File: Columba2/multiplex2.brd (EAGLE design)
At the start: 37.7 x 35.1 mm, 19 parts, among them U1 MAX4617CUE+T

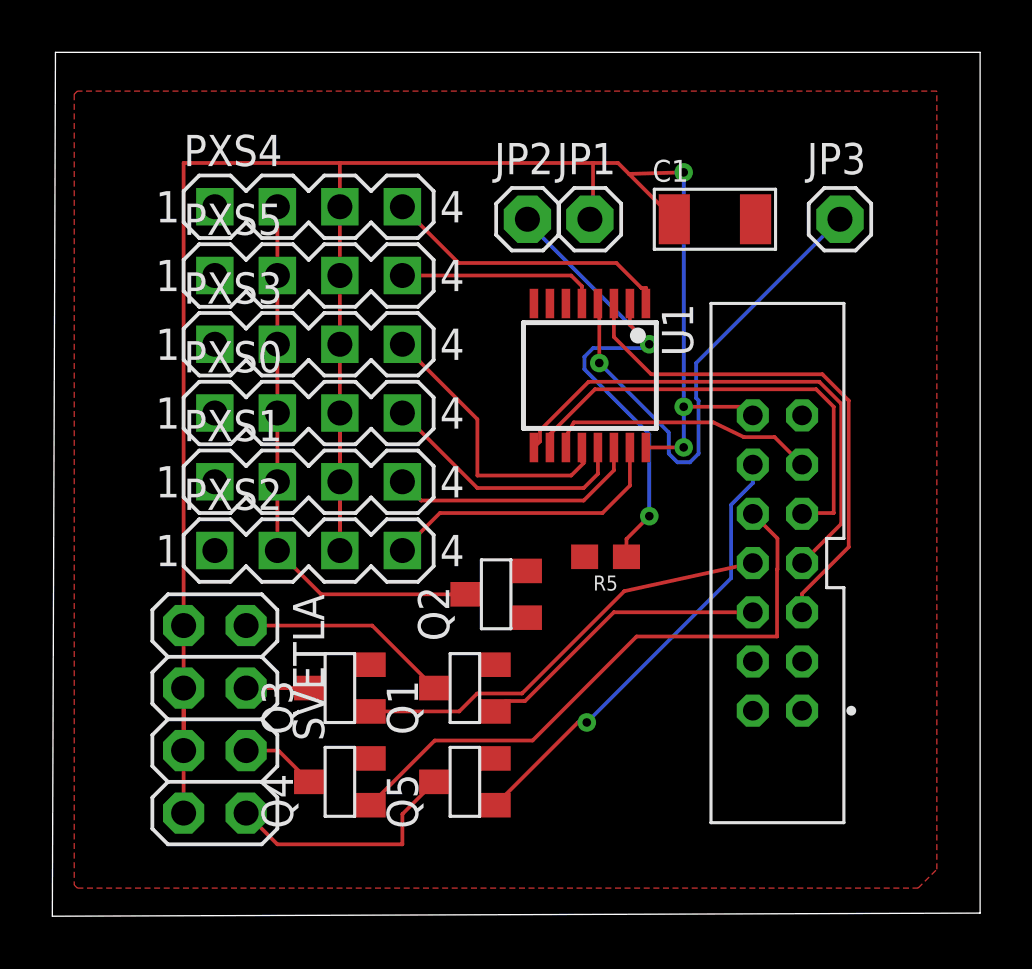
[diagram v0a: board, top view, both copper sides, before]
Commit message: Add files via upload
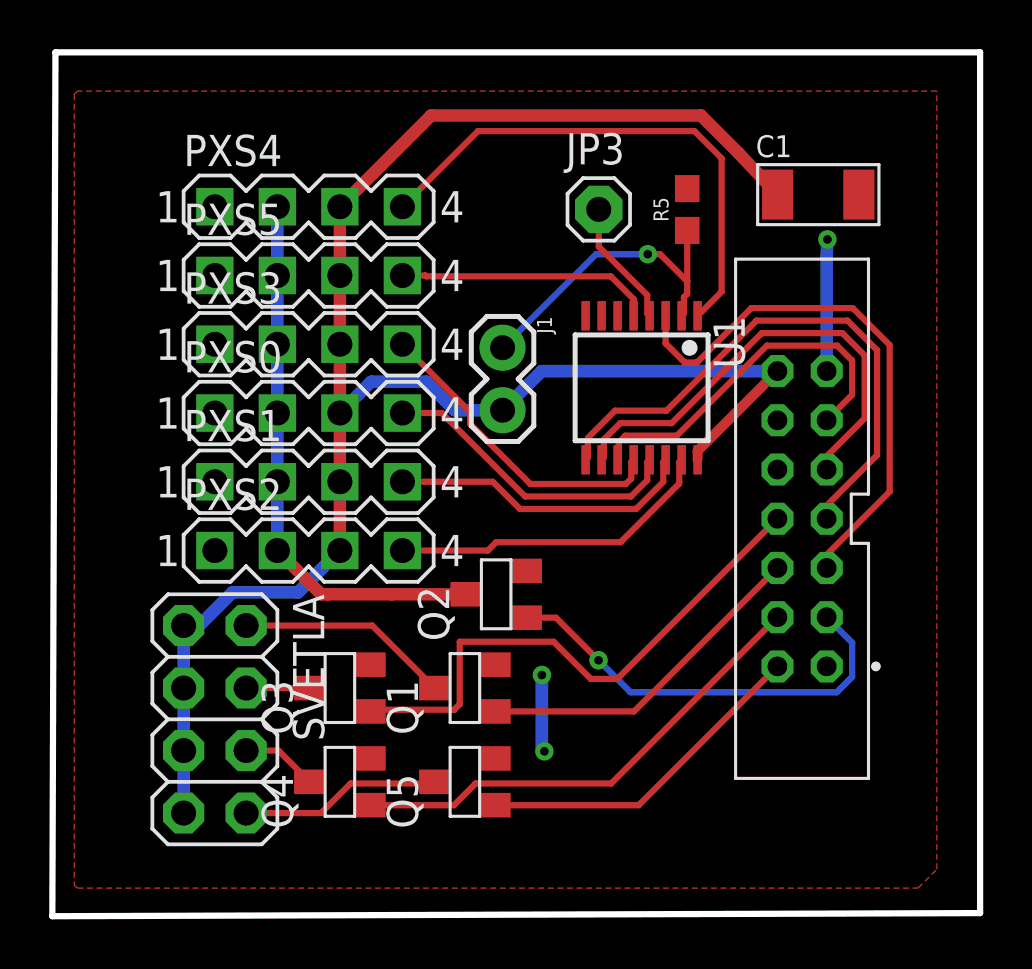
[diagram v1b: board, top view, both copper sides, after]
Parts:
- removed JP1, JP2: (no value), adafruit:1X01
- added J1: LIGHT, SparkFun-Connectors:1X02
- JP3: value (none) -> extra
- moved R5 14.5 mm to (23.0, 96.9), turned to 90 degrees
- moved JP3 9.81 mm to (19.4, 96.9)
- moved C1 4.32 mm to (28.3, 97.5)
- moved U1 2.16 mm to (21.1, 89.7)
- moved JL1 2.06 mm to (27.7, 84.3)
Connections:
- net 5V: now also J1.2; no longer JP1.1
- net LIGHT_S: now also J1.1; no longer JP2.1
- net PX_EN: now also JL1.P$3
- net SV0: now also JL1.P$2; no longer JL1.P$12
- net SV1: now also JL1.P$4; no longer JL1.P$10
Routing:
- net PX_EN: track 0.00 -> 17.6 mm, vias 0 -> 1
- net 5V: track 91.4 -> 74.3 mm, vias 3 -> 0
- net N$8: track 20.8 -> 5.18 mm, vias 1 -> 0
- net PX4: track 11.9 -> 21.5 mm
- net LIGHT_S: track 21.7 -> 13.1 mm, vias 2 -> 1
- net GND: track 0.00 -> 8.49 mm, vias 0 -> 3
- net SV1: track 24.8 -> 19.7 mm
- net SV2: track 17.7 -> 22.5 mm
- net SV0: track 18.4 -> 13.8 mm, vias 1 -> 0
- net A: track 11.0 -> 14.9 mm
- net PX5: track 8.18 -> 10.5 mm
- net PX1: track 10.3 -> 12.4 mm
- net PX0: track 10.5 -> 12.5 mm
- net N$4: track 9.96 -> 8.19 mm
- net SV3: track 12.1 -> 13.9 mm
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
